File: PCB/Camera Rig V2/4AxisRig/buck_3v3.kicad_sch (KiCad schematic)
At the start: 9 parts, among them U3 AN_SY8105

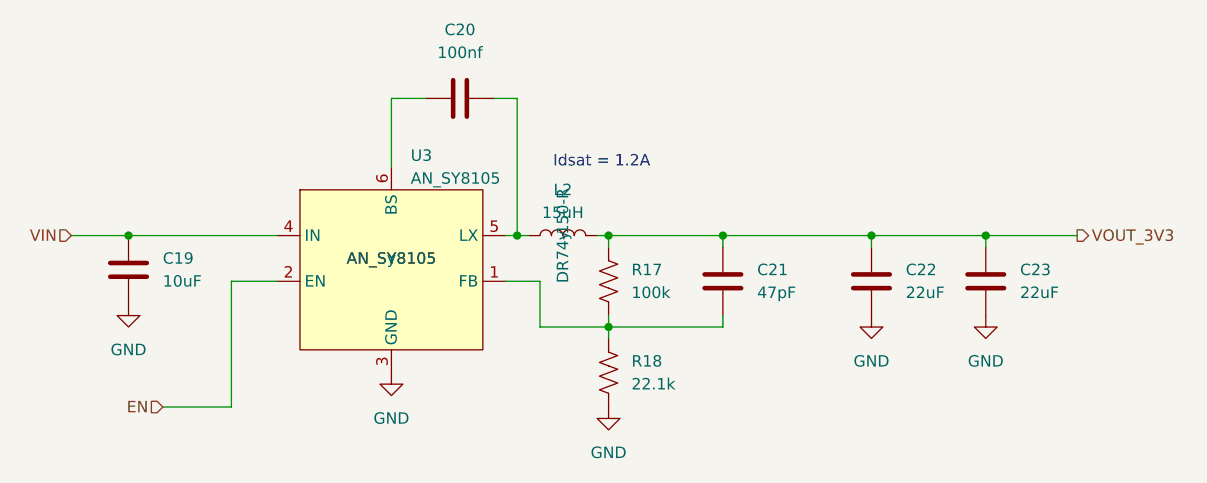
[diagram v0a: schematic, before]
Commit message: PCB V2 first draft
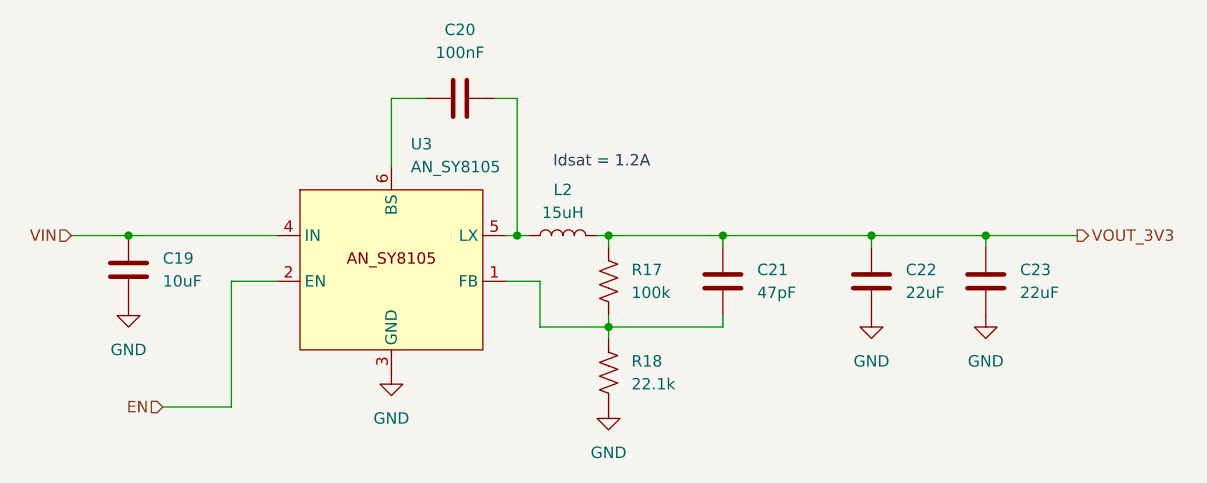
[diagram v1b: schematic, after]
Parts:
- C19, C21: footprint (none) -> Capacitor_SMD:C_0603_1608Metric_Pad1.08x0.95mm_HandSolder
- C20: value 100nf -> 100nF; footprint (none) -> Capacitor_SMD:C_0603_1608Metric_Pad1.08x0.95mm_HandSolder
- C22, C23: footprint (none) -> Capacitor_SMD:C_1206_3216Metric_Pad1.33x1.80mm_HandSolder
- L2, U3: Unique FP y -> (none)
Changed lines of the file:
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@@
 			)
 		)
-		(property "Footprint" ""
+		(property "Footprint" "Capacitor_SMD:C_0603_1608Metric_Pad1.08x0.95mm_HandSolder"
 			(at 98.7552 93.98 0)
 			(effects
@@
 			)
 		)
-		(property "Unique FP" ""
-			(at 97.79 90.17 0)
-			(effects
-				(font
-					(size 1.27 1.27)
-				)
-			)
-		)
 		(pin "1"
 		)
@@
 			)
 		)
-		(property "Footprint" ""
+		(property "Footprint" "Capacitor_SMD:C_1206_3216Metric_Pad1.33x1.80mm_HandSolder"
 			(at 181.3052 95.25 0)
 			(effects
@@
 			)
 		)
-		(property "Datasheet" "~"
+		(property "Datasheet" "https://mm.digikey.com/Volume0/opasdata/d220001/medias/docus/506/TMK316BBJ226ML-T_SS.pdf"
 			(at 180.34 91.44 0)
 			(effects
@@
 			)
 		)
-		(property "Unique FP" ""
-			(at 180.34 91.44 0)
-			(effects
-				(font
-					(size 1.27 1.27)
-				)
-			)
-		)
 		(pin "1"
 		)
@@
 			)
 		)
-		(property "Unique FP" ""
-			(at 151.13 101.6 0)
-			(effects
-				(font
-					(size 1.27 1.27)
-				)
-			)
-		)
 		(pin "2"
 		)
@@
 		(fields_autoplaced yes)
 		(property "Reference" "U3"
-			(at 129.1433 77.47 0)
+			(at 129.1433 76.2 0)
 			(effects
 				(font
@@
 		)
 		(property "Value" "AN_SY8105"
-			(at 129.1433 80.01 0)
+			(at 129.1433 78.74 0)
 			(effects
 				(font
@@
 					(size 1.27 1.27)
 				)
-			)
-		)
-		(property "Unique FP" "y"
-			(at 127 88.9 0)
-			(effects
-				(font
-					(size 1.27 1.27)
-				)
+				(hide yes)
 			)
 		)
@@
 			)
 		)
-		(property "Footprint" ""
+		(property "Footprint" "Capacitor_SMD:C_0603_1608Metric_Pad1.08x0.95mm_HandSolder"
 			(at 164.7952 95.25 0)
 			(effects
@@
 			)
 		)
-		(property "Unique FP" ""
-			(at 163.83 91.44 0)
-			(effects
-				(font
-					(size 1.27 1.27)
-				)
-			)
-		)
 		(pin "1"
 		)
@@
 					(size 1.27 1.27)
 				)
-			)
-		)
-		(property "Unique FP" "y"
-			(at 146.05 86.36 0)
-			(effects
-				(font
-					(size 1.27 1.27)
-				)
+				(hide yes)
 			)
 		)
@@
 			)
 		)
-		(property "Footprint" ""
+		(property "Footprint" "Capacitor_SMD:C_1206_3216Metric_Pad1.33x1.80mm_HandSolder"
 			(at 194.0052 95.25 0)
 			(effects
@@
 			)
 		)
-		(property "Datasheet" "~"
+		(property "Datasheet" "https://mm.digikey.com/Volume0/opasdata/d220001/medias/docus/506/TMK316BBJ226ML-T_SS.pdf"
 			(at 193.04 91.44 0)
 			(effects
@@
 			)
 		)
-		(property "Unique FP" ""
-			(at 193.04 91.44 0)
-			(effects
-				(font
-					(size 1.27 1.27)
-				)
-			)
-		)
 		(pin "1"
 		)
@@
 			)
 		)
-		(property "Unique FP" ""
-			(at 151.13 91.44 0)
-			(effects
-				(font
-					(size 1.27 1.27)
-				)
-			)
-		)
 		(pin "2"
 		)
@@
 			)
 		)
-		(property "Value" "100nf"
+		(property "Value" "100nF"
 			(at 134.62 66.04 90)
 			(effects
@@
 			)
 		)
-		(property "Footprint" ""
+		(property "Footprint" "Capacitor_SMD:C_0603_1608Metric_Pad1.08x0.95mm_HandSolder"
 			(at 130.81 72.0852 0)
 			(effects
@@
 			(at 134.62 71.12 0)
 			(effects
-				(font
-					(size 1.27 1.27)
-				)
-			)
-		)
-		(property "Unique FP" ""
-			(at 134.62 71.12 0)
-			(effects
